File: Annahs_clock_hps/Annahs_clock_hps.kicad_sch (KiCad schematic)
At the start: 19 parts, among them J1 PJ-102AH, Y1 Crystal 22p

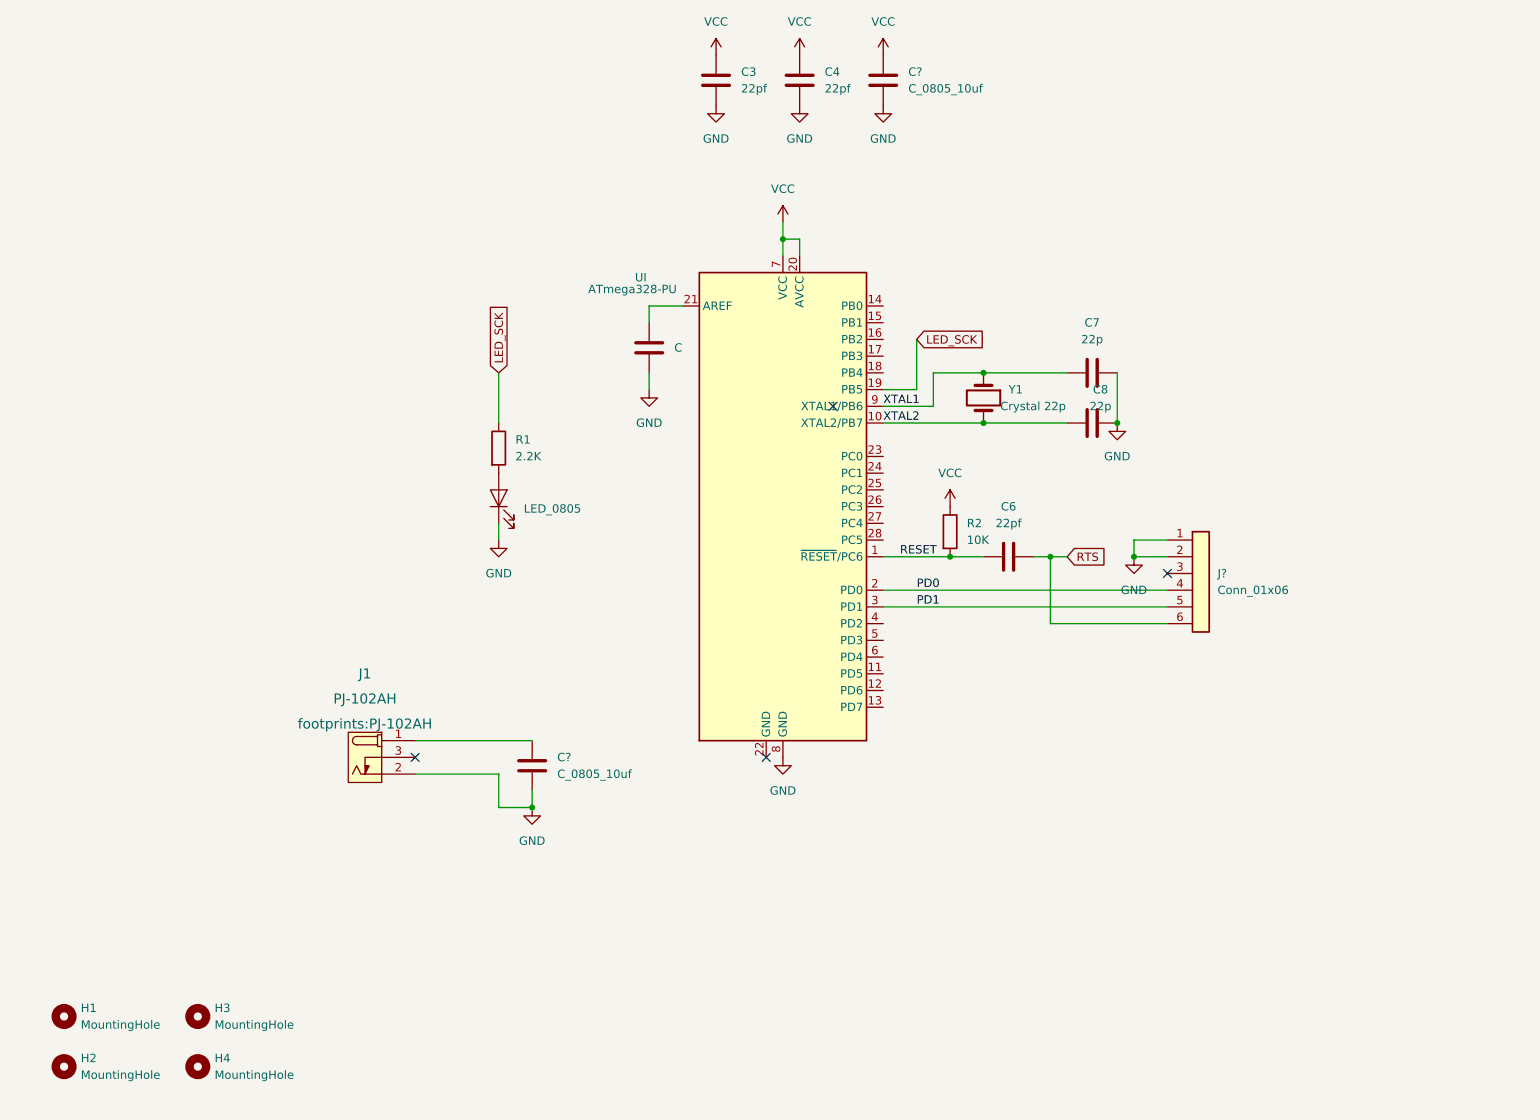
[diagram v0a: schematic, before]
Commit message: Clock Schematic
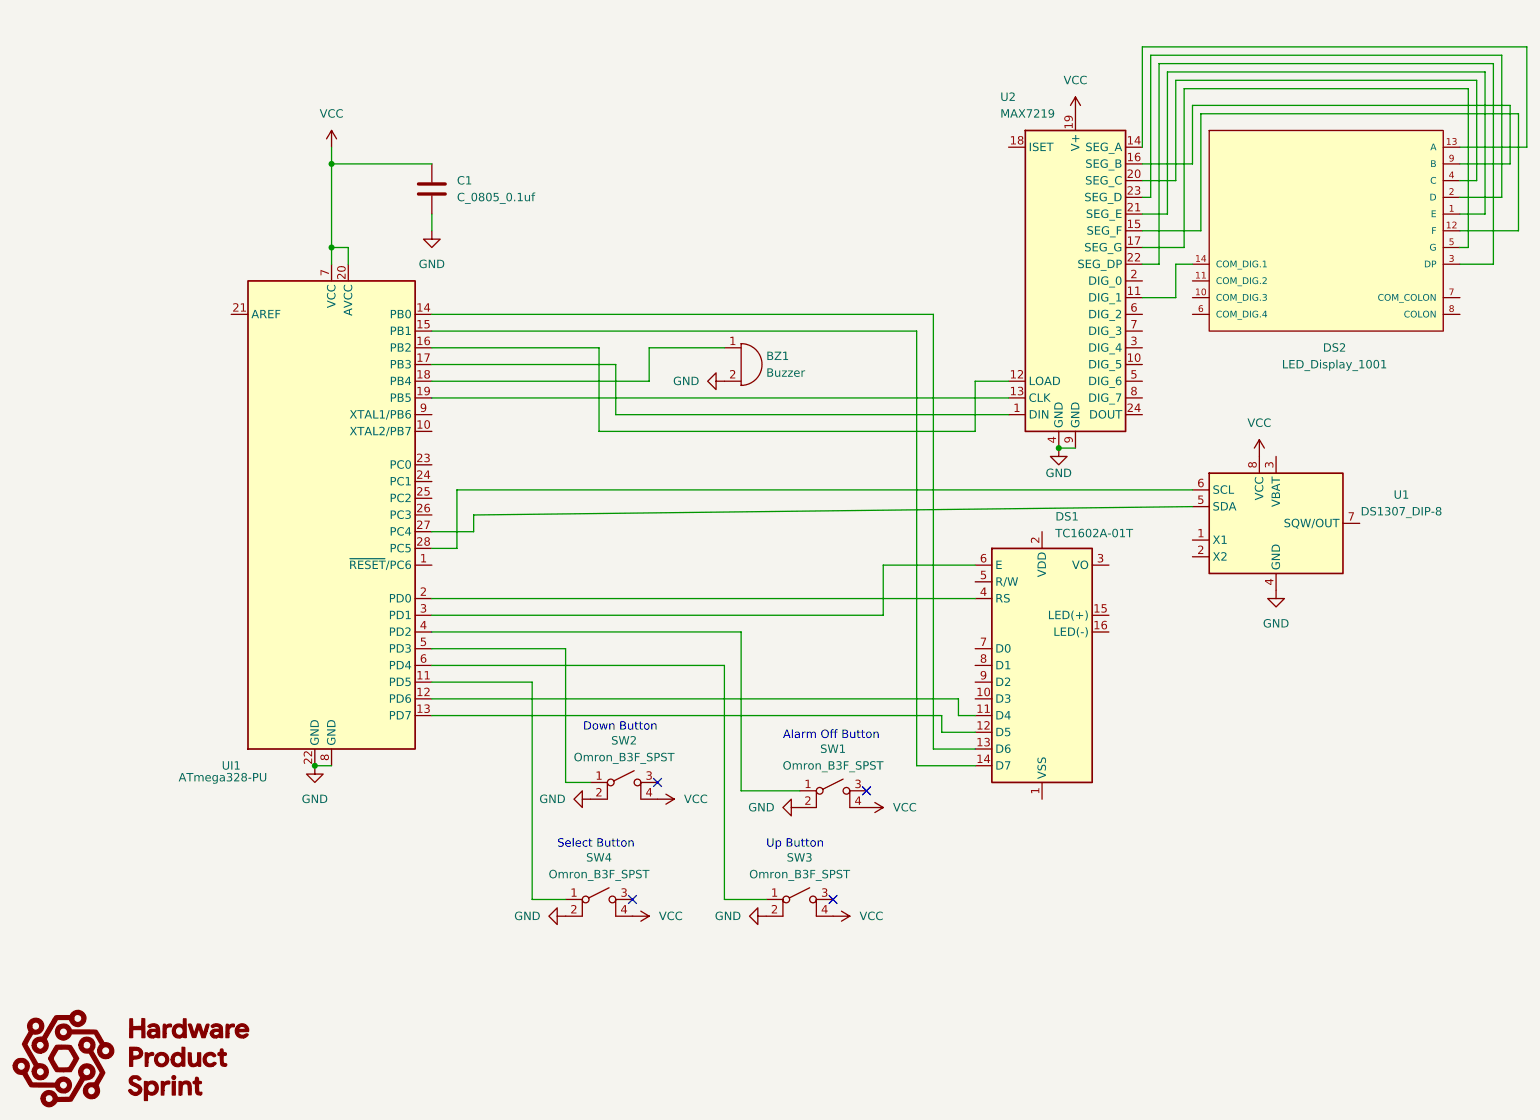
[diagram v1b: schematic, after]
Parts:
- removed C: C_0805_22pf, footprints:C_0805_2012Metric, symbol HPS:C_0805_22pf
- removed C3, C4, C6: 22pf, footprints:C_0805_2012Metric, symbol HPS:C_0805_22pf
- removed C7, C8: 22p, footprints:C_0805_2012Metric, symbol HPS:C_0805_22pf
- removed C? (x2): C_0805_10uf, footprints:C_0805_2012Metric, symbol HPS:C_0805_10uf
- removed D?: LED_0805, footprints:LED_0805_2012Metric, symbol HPS:LED_0805
- removed H1, H2, H3, H4: MountingHole, footprints:MountingHole_3.2mm_M3, symbol HPS:MountingHole
- removed J1: PJ-102AH, footprints:PJ-102AH, symbol HPS:PJ-102AH
- removed J?: Conn_01x06, footprints:PinHeader_1x06_P2.54mm_Vertical, symbol HPS:Conn_01x06
- removed R1: 2.2K, footprints:R_0805_2012Metric, symbol HPS:R_0805_2.2K
- removed R2: 10K, footprints:R_0805_2012Metric, symbol HPS:R_0805_10K
- removed Y1: Crystal 22p, footprints:Crystal_SMD_HC49-SD, symbol HPS:Crystal_16MHz
- added BZ1: Buzzer, footprints:Buzzer_TDK_PS1240P02BT_D12.2mm_H6.5mm, symbol HPS:Buzzer
- added C1: C_0805_0.1uf, footprints:C_0805_2012Metric, symbol HPS:C_0805_0.1uf
- added DS1: TC1602A-01T, footprints:TC1602A-01T, symbol HPS:TC1602A-01T
- added DS2: LED_Display_1001, footprints:Adafruit-1001-0-0-MFG, symbol HPS:LED_Display_1001
- added SW1, SW2, SW3, SW4: Omron_B3F_SPST, footprints:SW_SPST_Omron_B3FS-100xP, symbol HPS_3:Omron_B3F_SPST
- added U1: DS1307_DIP-8, footprints:DIP-8_W7.62mm, symbol HPS:DS1307_DIP-8
- added U2: MAX7219, footprints:DIP-24_W7.62mm, symbol HPS:MAX7219
- renumbered UI to UI1
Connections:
- net GND: now also UI1.22 (GND), BZ1.2 (+), C1.2, SW1.2 (A), SW2.2 (A), SW3.2 (A), SW4.2 (A), U1.4 (GND), U2.4 (GND), U2.9 (GND)
- net VCC: now also C1.1, SW1.4 (B), SW2.4 (B), SW3.4 (B), SW4.4 (B), U1.8 (VCC), U2.19 (V+)
- net at UI1.11 (PD5): now also SW4.1 (A)
- net at UI1.12 (PD6): now also DS1.11 (D4)
- net at UI1.13 (PD7): now also DS1.12 (D5)
- net at UI1.14 (PB0): now also DS1.13 (D6)
- net at UI1.15 (PB1): now also DS1.14 (D7)
- net at UI1.16 (PB2): now also U2.12 (LOAD)
- net at UI1.17 (PB3): now also U2.1 (DIN)
- net at UI1.18 (PB4): now also BZ1.1 (-)
- net at UI1.27 (PC4): now also U1.5 (SDA)
- net at UI1.28 (PC5): now also U1.6 (SCL)
- net at UI1.4 (PD2): now also SW1.1 (A)
- net at UI1.5 (PD3): now also SW2.1 (A)
- net at UI1.6 (PD4): now also SW3.1 (A)
- net LED_SCK: no longer names the net of UI1.19 (PB5)
- net LED_SCK: now also U2.13 (CLK)
- net PD0: no longer names the net of UI1.2 (PD0)
- net PD0: now also DS1.4 (RS)
- net PD1: no longer names the net of UI1.3 (PD1)
- net PD1: now also DS1.6 (E)
- net RESET: no longer names the net of UI1.1 (~{RESET}/PC6)
- net XTAL1: no longer names the net of UI1.9 (XTAL1/PB6)
- net XTAL2: no longer names the net of UI1.10 (XTAL2/PB7)
- new net: DS2.1 (E), U2.21 (SEG_E)
- new net: DS2.12 (F), U2.15 (SEG_F)
- new net: DS2.13 (A), U2.14 (SEG_A)
- new net: DS2.14 (COM_DIG.1), U2.11 (DIG_1)
- new net: DS2.2 (D), U2.23 (SEG_D)
- new net: DS2.3 (DP), U2.22 (SEG_DP)
- new net: DS2.4 (C), U2.20 (SEG_C)
- new net: DS2.5 (G), U2.17 (SEG_G)
- new net: DS2.9 (B), U2.16 (SEG_B)
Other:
- note added: "Alarm Off Button"
- note added: "Down Button"
- note added: "Select Button"
- note added: "Up Button"
- moved on the sheet: UI1
